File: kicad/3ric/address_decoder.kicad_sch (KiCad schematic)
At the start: 40 parts

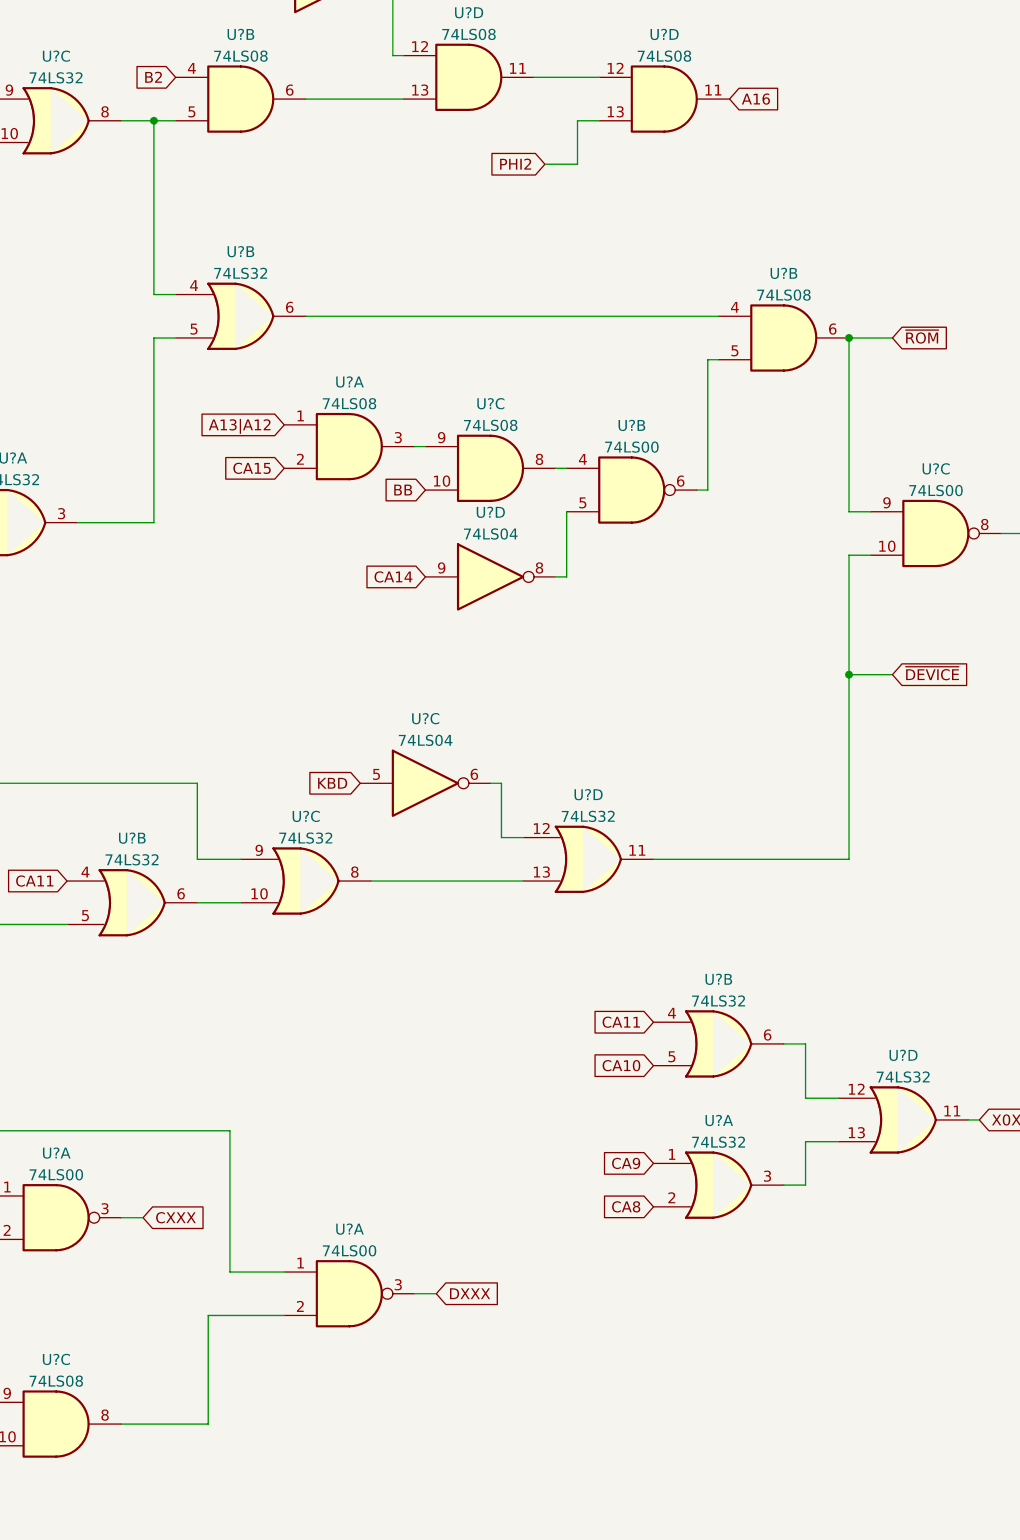
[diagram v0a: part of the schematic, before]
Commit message: schematic updates
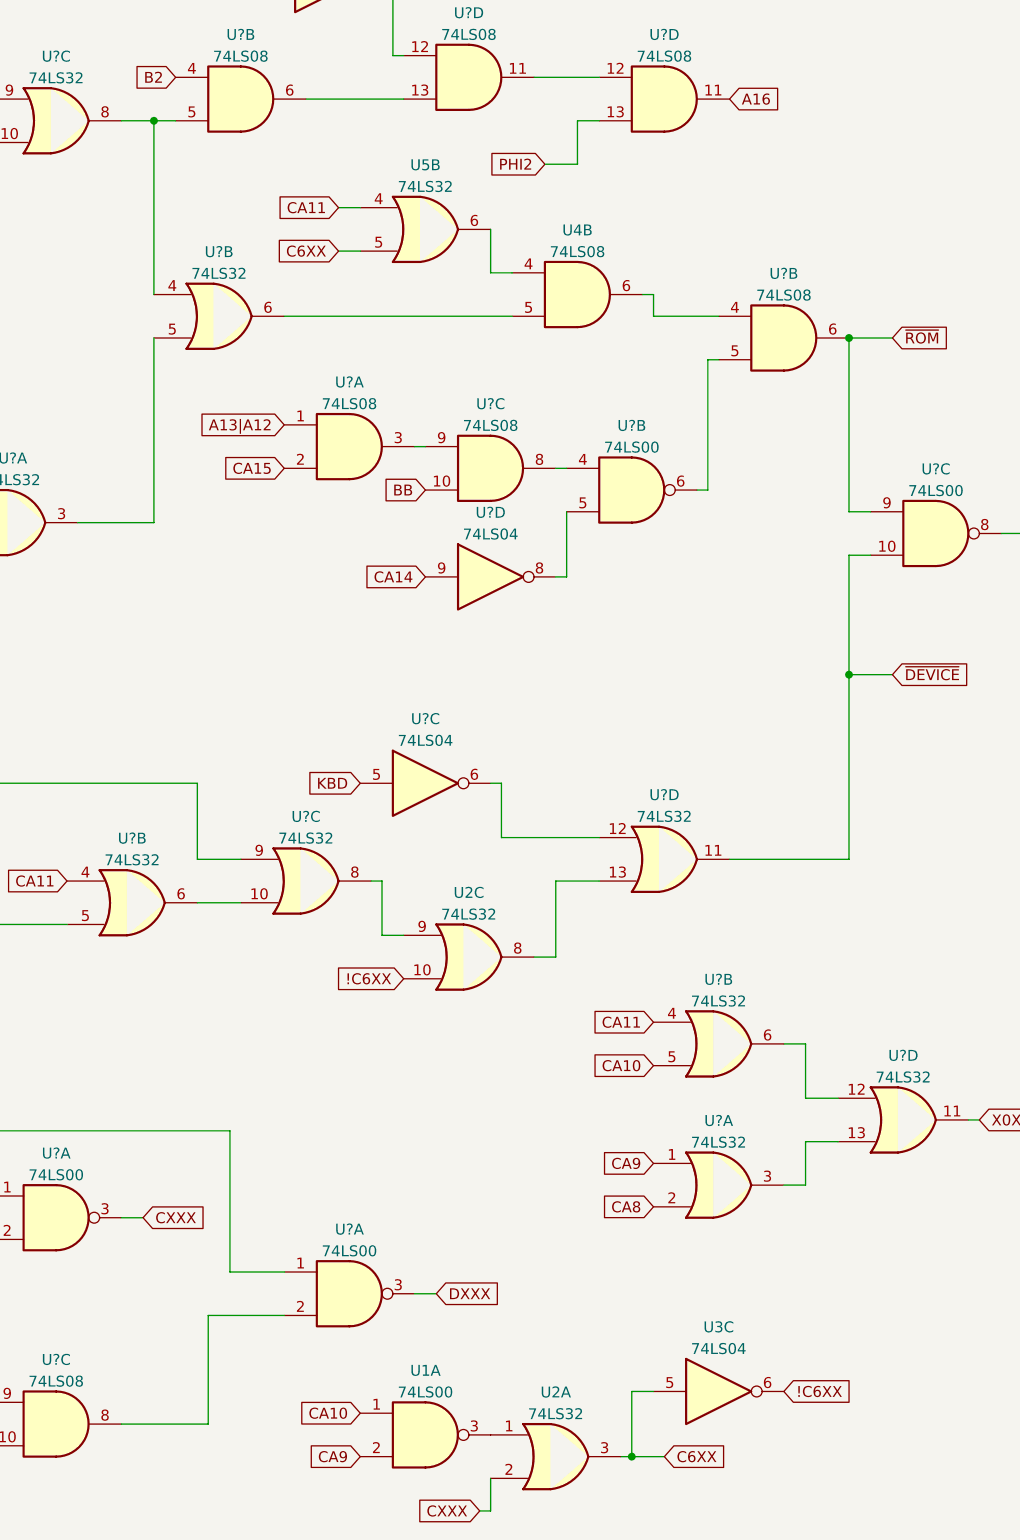
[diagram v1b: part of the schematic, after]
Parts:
- added U1: 74LS00, symbol 74xx:74LS00
- added U2, U5: 74LS32, symbol 74xx:74LS32
- added U3: 74LS04, symbol 74xx:74LS04
- added U4: 74LS08, symbol 74xx:74LS08
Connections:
- net CA10: now also U1.1
- net CA11: now also U5.4
- net CA9: now also U1.2
- net CXXX: now also U2.2
- net at U?.13: now also U2.8; no longer U?.8
- net at U?.6: now also U4.5; no longer U?.4
- new net: U1.3, U2.1
- new net: U2.9, U?.8
- new net: U4.4, U5.6
- new net: U4.6, U?.4
- new net !C6XX: U2.10, U3.6
- new net C6XX: U2.3, U3.5, U5.5
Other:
- moved on the sheet: U?B, U?D
